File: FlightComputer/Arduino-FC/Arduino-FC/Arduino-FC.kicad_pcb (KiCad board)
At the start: 2 copper layers, 95 x 86.9 mm, 30 parts, among them J1 Conn_01x04, J2 Conn_01x08, J3 Conn_01x06, J4 Conn_01x03, J5 Screw_Terminal_01x02, J6 Conn_01x02, J7 Conn_01x02, U1 NRF24L01_Breakout

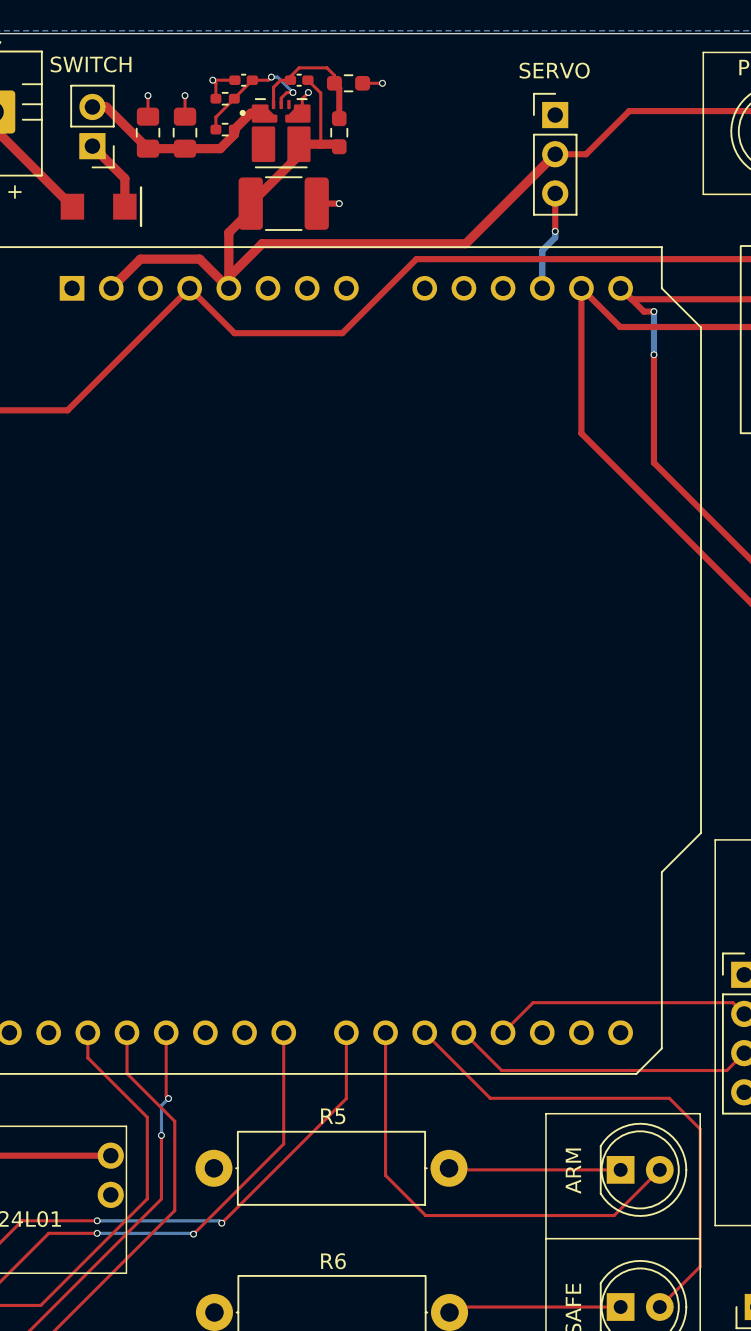
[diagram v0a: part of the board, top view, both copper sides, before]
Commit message: DRC Resolutions
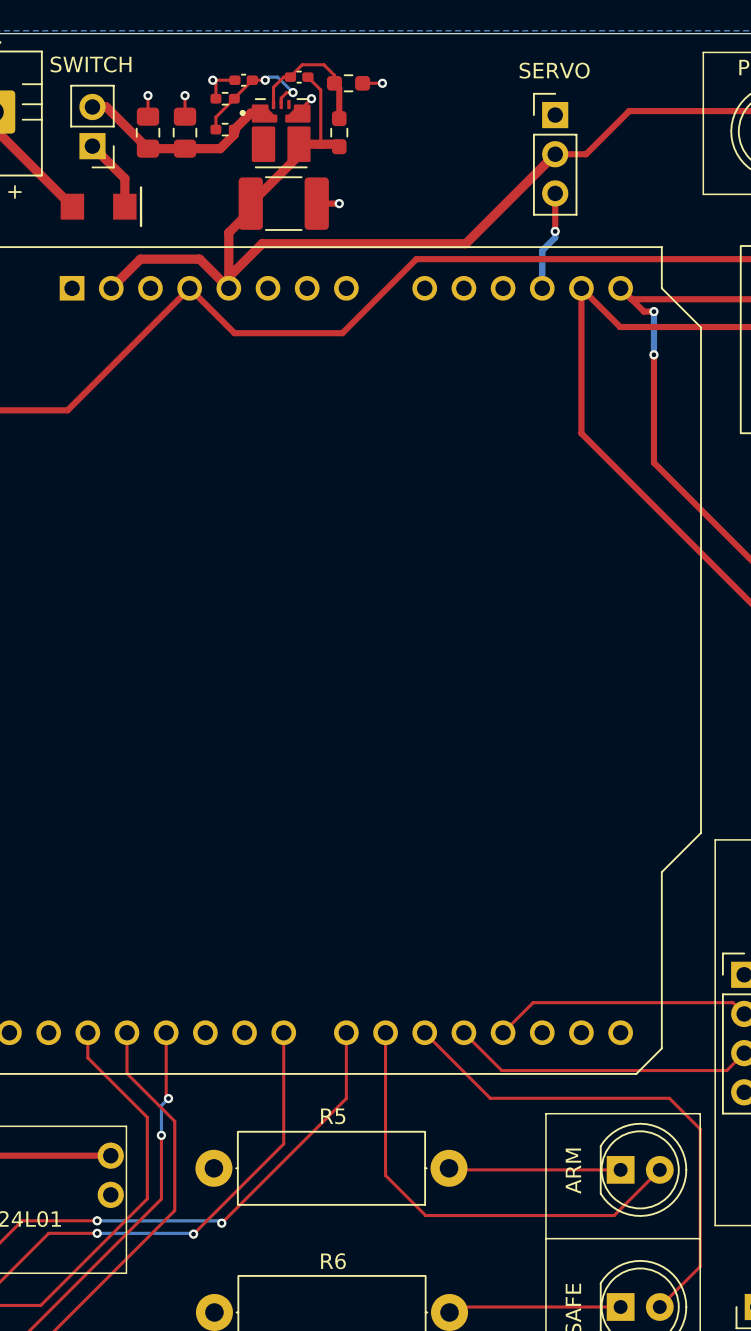
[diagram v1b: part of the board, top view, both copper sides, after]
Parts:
- moved C4 0.20 mm to (146.8, 46.0)
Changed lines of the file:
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@@
 	(footprint "Capacitor_SMD:C_0402_1005Metric_Pad0.74x0.62mm_HandSolder"
 		(layer "F.Cu")
-		(at 146.8 46.2 180)
+		(at 146.8 46 180)
 		(descr "Capacitor SMD 0402 (1005 Metric), square (rectangular) end terminal, IPC-7351 nominal with elongated pad for handsoldering. (Body size source: IPC-SM-782 page 76, https://www.pcb-3d.com/wordpress/wp-content/uploads/ipc-sm-782a_amendment_1_and_2.pdf), generated with kicad-footprint-generator")
 		(tags "capacitor handsolder")
@@
 	)
 	(segment
-		(start 147 47.4)
-		(end 147.4 47)
-		(width 0.2)
-		(layer "F.Cu")
-		(net 3)
-	)
-	(segment
 		(start 141.4025 47.4)
 		(end 141.4025 46.4025)
@@
 	)
 	(segment
-		(start 147 48.3375)
-		(end 147 47.4)
-		(width 0.2)
-		(layer "F.Cu")
-		(net 3)
-	)
-	(segment
 		(start 142.6325 46.2)
 		(end 141.2 46.2)
@@
 	)
 	(segment
+		(start 147.6 47.4)
+		(end 147 48)
+		(width 0.2)
+		(layer "F.Cu")
+		(net 3)
+	)
+	(segment
 		(start 147.9375 54.2)
 		(end 149.4 54.2)
@@
 	)
 	(segment
+		(start 147 48)
+		(end 147 48.3375)
+		(width 0.2)
+		(layer "F.Cu")
+		(net 3)
+	)
+	(segment
 		(start 150.9125 46.4)
 		(end 152.2 46.4)
@@
 	(via
 		(at 152.2 46.4)
-		(size 0.45)
+		(size 0.6)
 		(drill 0.3)
 		(layers "F.Cu" "B.Cu")
@@
 	(via
 		(at 139.4 47.2)
-		(size 0.45)
+		(size 0.6)
 		(drill 0.3)
 		(layers "F.Cu" "B.Cu")
@@
 	(via
 		(at 149.4 54.2)
-		(size 0.45)
+		(size 0.6)
 		(drill 0.3)
 		(layers "F.Cu" "B.Cu")
@@
 	(via
 		(at 137 47.2)
-		(size 0.45)
+		(size 0.6)
 		(drill 0.3)
 		(layers "F.Cu" "B.Cu")
@@
 	(via
 		(at 141.2 46.2)
-		(size 0.45)
+		(size 0.6)
 		(drill 0.3)
 		(layers "F.Cu" "B.Cu")
@@
 	)
 	(via
-		(at 147.4 47)
-		(size 0.45)
+		(at 147.6 47.4)
+		(size 0.6)
 		(drill 0.3)
 		(layers "F.Cu" "B.Cu")
@@
 	(via
 		(at 169.8 61.2)
-		(size 0.45)
+		(size 0.6)
 		(drill 0.3)
 		(layers "F.Cu" "B.Cu")
@@
 	(via
 		(at 169.8 64)
-		(size 0.45)
+		(size 0.6)
 		(drill 0.3)
 		(layers "F.Cu" "B.Cu")
@@
 	(via
 		(at 163.4 56)
-		(size 0.45)
+		(size 0.6)
 		(drill 0.3)
 		(layers "F.Cu" "B.Cu")
@@
 	(via
 		(at 139.954 121.0056)
-		(size 0.45)
+		(size 0.6)
 		(drill 0.3)
 		(layers "F.Cu" "B.Cu")
@@
 	(via
 		(at 133.7056 120.9548)
-		(size 0.45)
+		(size 0.6)
 		(drill 0.3)
 		(layers "F.Cu" "B.Cu")
@@
 	)
 	(segment
-		(start 148.2 47.0325)
-		(end 148.2 50.35)
-		(width 0.2)
-		(layer "F.Cu")
-		(net 15)
-	)
-	(segment
 		(start 168.2 48.2)
 		(end 177.74 48.2)
@@
 	)
 	(segment
+		(start 147.3675 46.2)
+		(end 147.5675 46.2)
+		(width 0.2)
+		(layer "F.Cu")
+		(net 15)
+	)
+	(segment
 		(start 189.46 48.26)
 		(end 177.8 48.26)
@@
 	)
 	(segment
-		(start 147.3675 46.2)
-		(end 148.2 47.0325)
-		(width 0.2)
-		(layer "F.Cu")
-		(net 15)
-	)
-	(segment
 		(start 134.62 59.69)
 		(end 136.51 57.8)
@@
 	)
 	(segment
+		(start 148.2 46.8325)
+		(end 148.2 50.35)
+		(width 0.2)
+		(layer "F.Cu")
+		(net 15)
+	)
+	(segment
 		(start 142.24 58.96)
 		(end 142.24 59.69)
@@
 	)
 	(segment
+		(start 147.5675 46.2)
+		(end 148.2 46.8325)
+		(width 0.2)
+		(layer "F.Cu")
+		(net 15)
+	)
+	(segment
 		(start 146.7875 50.35)
 		(end 148.2 50.35)
@@
 	(via
 		(at 138.3284 112.2172)
-		(size 0.45)
+		(size 0.6)
 		(drill 0.3)
 		(layers "F.Cu" "B.Cu")
@@
 	(via
 		(at 137.8712 114.6048)
-		(size 0.45)
+		(size 0.6)
 		(drill 0.3)
 		(layers "F.Cu" "B.Cu")
@@
 	(via
 		(at 133.7056 120.142)
-		(size 0.45)
+		(size 0.6)
 		(drill 0.3)
 		(layers "F.Cu" "B.Cu")
@@
 	(via
 		(at 141.7828 120.2944)
-		(size 0.45)
+		(size 0.6)
 		(drill 0.3)
 		(layers "F.Cu" "B.Cu")
@@
 	)
 	(segment
-		(start 144.8 46.2)
-		(end 145 46)
-		(width 0.2)
-		(layer "F.Cu")
-		(net 28)
-	)
-	(segment
 		(start 142.5975 47.37)
 		(end 143.7675 46.2)
@@
 	)
 	(segment
+		(start 146 47)
+		(end 145.6375 47.3625)
+		(width 0.2)
+		(layer "F.Cu")
+		(net 28)
+	)
+	(segment
+		(start 141.4025 48.595)
+		(end 142.5975 47.4)
+		(width 0.2)
+		(layer "F.Cu")
+		(net 28)
+	)
+	(segment
+		(start 144.6 46.2)
+		(end 143.7675 46.2)
+		(width 0.2)
+		(layer "F.Cu")
+		(net 28)
+	)
+	(segment
+		(start 141.4025 49.4)
+		(end 141.4025 48.595)
+		(width 0.2)
+		(layer "F.Cu")
+		(net 28)
+	)
+	(segment
 		(start 145.6375 47.3625)
 		(end 145.6375 47.775)
@@
 	)
 	(segment
-		(start 141.4025 48.595)
-		(end 142.5975 47.4)
-		(width 0.2)
-		(layer "F.Cu")
-		(net 28)
-	)
-	(segment
-		(start 141.4025 49.4)
-		(end 141.4025 48.595)
-		(width 0.2)
-		(layer "F.Cu")
-		(net 28)
-	)
-	(segment
 		(start 142.5975 47.4)
 		(end 142.5975 47.37)
@@
 	)
 	(segment
-		(start 143.7675 46.2)
-		(end 144.8 46.2)
-		(width 0.2)
-		(layer "F.Cu")
-		(net 28)
-	)
-	(segment
-		(start 146 47)
-		(end 145.6375 47.3625)
-		(width 0.2)
-		(layer "F.Cu")
-		(net 28)
-	)
-	(segment
 		(start 146.4 47)
 		(end 146 47)
@@
 	(via
 		(at 146.4 47)
-		(size 0.45)
+		(size 0.6)
 		(drill 0.3)
 		(layers "F.Cu" "B.Cu")
@@
 	)
 	(via
-		(at 145 46)
-		(size 0.45)
+		(at 144.6 46.2)
+		(size 0.6)
 		(drill 0.3)
 		(layers "F.Cu" "B.Cu")
@@
 	)
 	(segment
-		(start 145 46)
+		(start 146.4 47)
 		(end 145.4 46)
 		(width 0.2)
@@
 	(segment
 		(start 145.4 46)
-		(end 146.4 47)
+		(end 144.8 46)
 		(width 0.2)
 		(layer "B.Cu")
@@
 	)
 	(segment
-		(start 146.2325 45.9675)
-		(end 146.8 45.4)
-		(width 0.2)
-		(layer "F.Cu")
-		(net 29)
-	)
-	(segment
-		(start 146.8 45.4)
-		(end 148.6 45.4)
-		(width 0.2)
-		(layer "F.Cu")
-		(net 29)
-	)
-	(segment
-		(start 148.6 45.4)
-		(end 149.0875 45.8875)
-		(width 0.2)
-		(layer "F.Cu")
-		(net 29)
-	)
-	(segment
-		(start 145.1375 46.6625)
-		(end 145.1375 47.775)
-		(width 0.2)
-		(layer "F.Cu")
-		(net 29)
-	)
-	(segment
-		(start 146.2325 46.2)
-		(end 145.6 46.2)
-		(width 0.2)
-		(layer "F.Cu")
-		(net 29)
+		(start 144.8 46)
+		(end 144.6 46.2)
+		(width 0.2)
+		(layer "B.Cu")
+		(net 28)
 	)
 	(segment
@@
 	)
 	(segment
-		(start 145.6 46.2)
+		(start 147 45.2)
+		(end 148.4 45.2)
+		(width 0.2)
+		(layer "F.Cu")
+		(net 29)
+	)
+	(segment
+		(start 146.2325 46)
+		(end 146.2325 45.9675)
+		(width 0.2)
+		(layer "F.Cu")
+		(net 29)
+	)
+	(segment
+		(start 145.1375 47.775)
 		(end 145.1375 46.6625)
+		(width 0.2)
+		(layer "F.Cu")
+		(net 29)
+	)
+	(segment
+		(start 148.4 45.2)
+		(end 149.0875 45.8875)
 		(width 0.2)
 		(layer "F.Cu")
@@
 	)
 	(segment
+		(start 145.8 46)
+		(end 146.2325 46)
+		(width 0.2)
+		(layer "F.Cu")
+		(net 29)
+	)
+	(segment
 		(start 149.4 48.6875)
 		(end 149.4 46.7125)
@@
 	)
 	(segment
-		(start 146.2325 46.2)
-		(end 146.2325 45.9675)
-		(width 0.2)
-		(layer "F.Cu")
+		(start 146.2325 45.9675)
+		(end 147 45.2)
+		(width 0.2)
+		(layer "F.Cu")
+		(net 29)
+	)
+	(segment
+		(start 145.1375 46.6625)
+		(end 145.8 46)
+		(width 0.2)
+		(layer "F.Cu")
